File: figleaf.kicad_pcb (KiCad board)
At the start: 2 copper layers, 145 x 105 mm, 70 parts, among them J1 Conn_01x02_Pin, J2 HRO_TYPE-C-31-M-14, J3 Battery, J9 TC2030_SWD, Q2 2N7002, SW1 PWR, SW2 RST, U1 SRV05-4, U10 MAX17048, U3 BQ24075, U8 nRF52840_moko_mk08

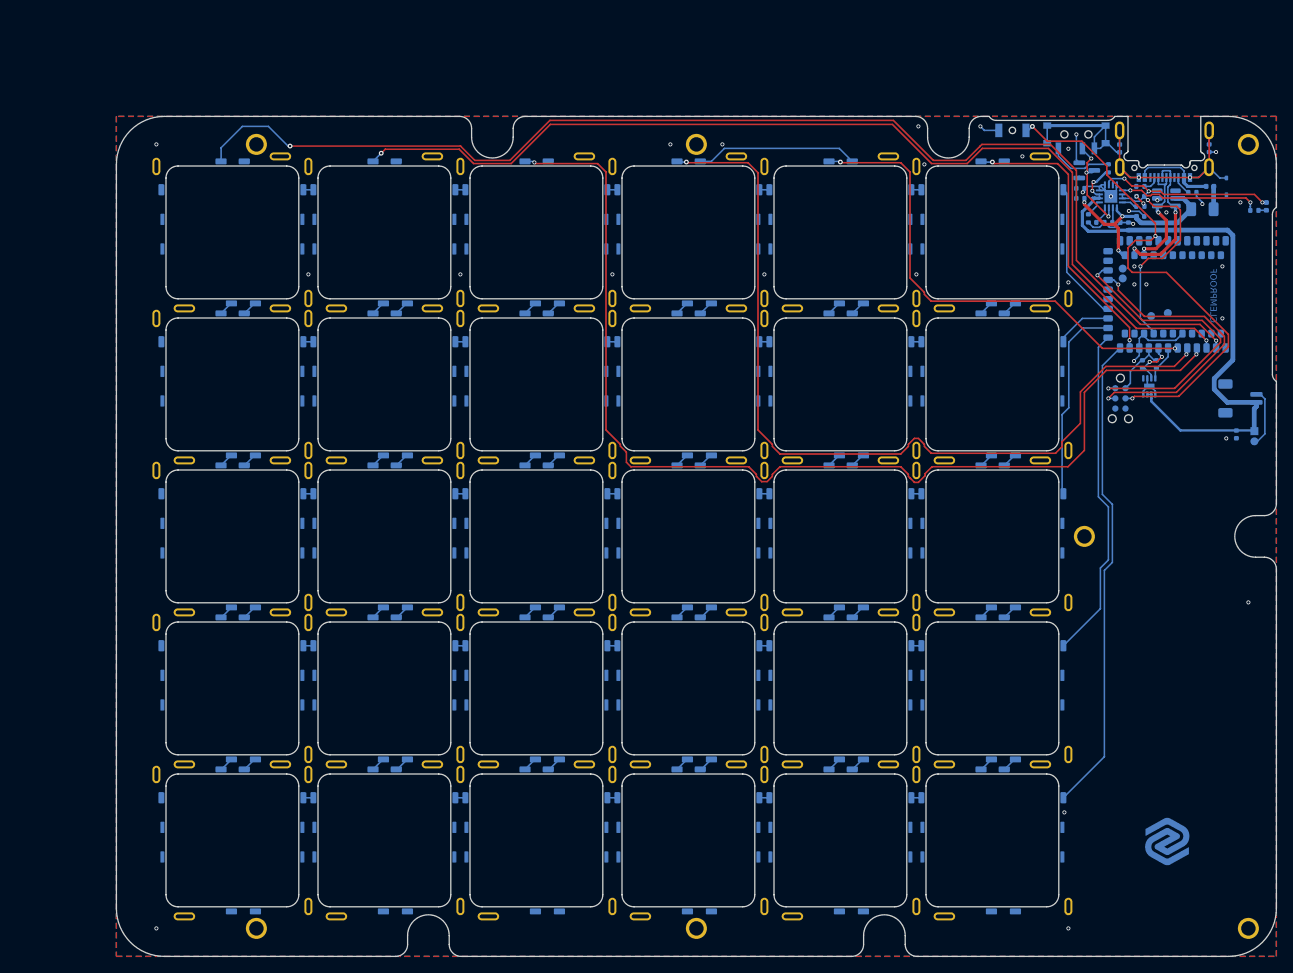
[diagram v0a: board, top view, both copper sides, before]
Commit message: Move XY to better coord
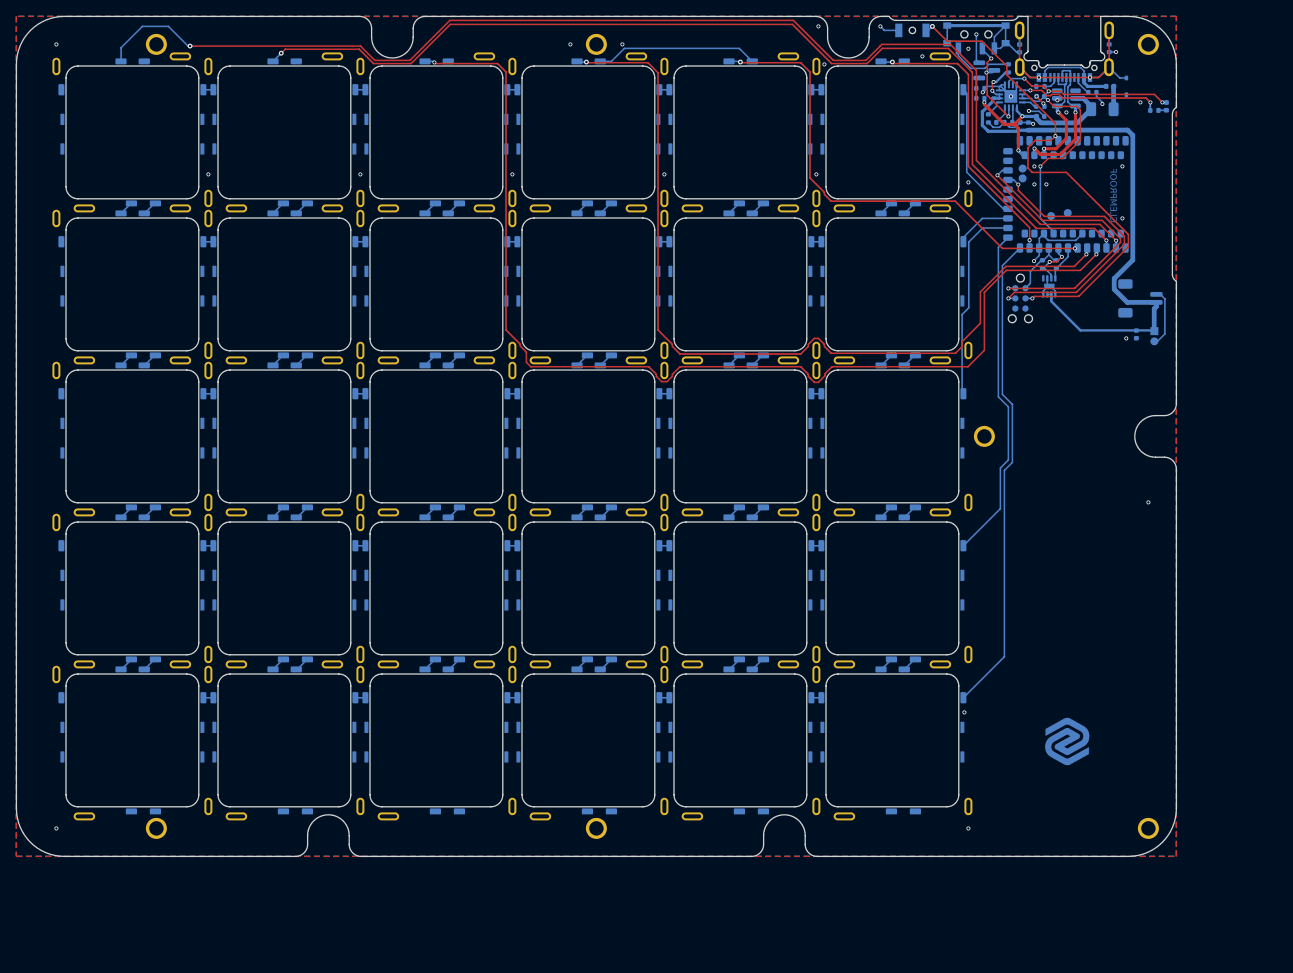
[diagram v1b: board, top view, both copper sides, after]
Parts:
- moved U8 17.7 mm to (134.2, 22.2)
- moved Q2 17.7 mm to (121.3, 6.75)
- moved C1 17.7 mm to (136.6, 3.98)
- moved C17 17.7 mm to (140.0, 39.8)
- moved C5 17.7 mm to (128.0, 12.5)
- moved C6 17.7 mm to (128.0, 10.0)
- moved C7 17.7 mm to (126.5, 13.8)
- moved D1 17.7 mm to (138.8, 8.75)
- moved F1 17.7 mm to (135.8, 11.6)
- moved H1 17.7 mm to (17.5, 3.50)
- moved H2 17.7 mm to (72.5, 3.50)
- moved H3 17.7 mm to (141.5, 3.50)
- moved H4 17.7 mm to (121.0, 52.5)
- moved H5 17.7 mm to (141.5, 101.5)
- moved H6 17.7 mm to (72.5, 101.5)
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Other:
- outline, holes or cut-outs redrawn
